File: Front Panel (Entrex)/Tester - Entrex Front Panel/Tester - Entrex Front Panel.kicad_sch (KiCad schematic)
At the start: 14 parts, among them J1 Conn_02x26_Top_Bottom, J1 Logic 8 CH, J11 Logic 8 CH, J12 Logic 8 CH, J2 Conn_01x04, J3 Conn_01x08, J4 Conn_01x08, J5 Conn_01x06, J6 Conn_01x04, J7 Conn_01x02, J8 Conn_01x19, J9 Logic 8 CH, SW1 SW_Push

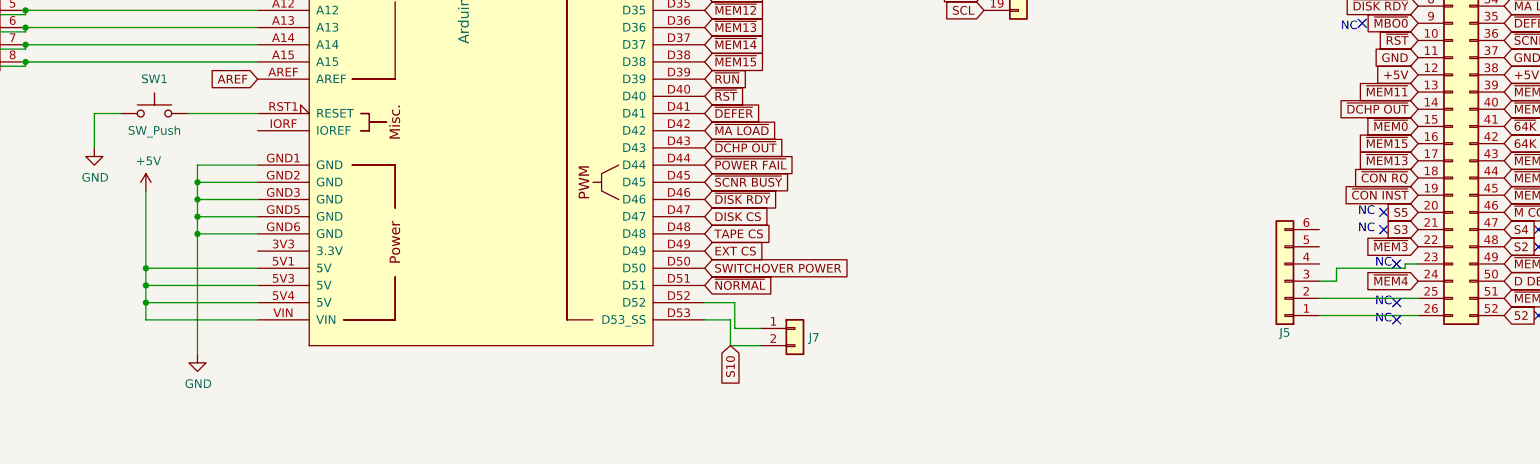
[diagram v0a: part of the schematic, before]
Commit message: build
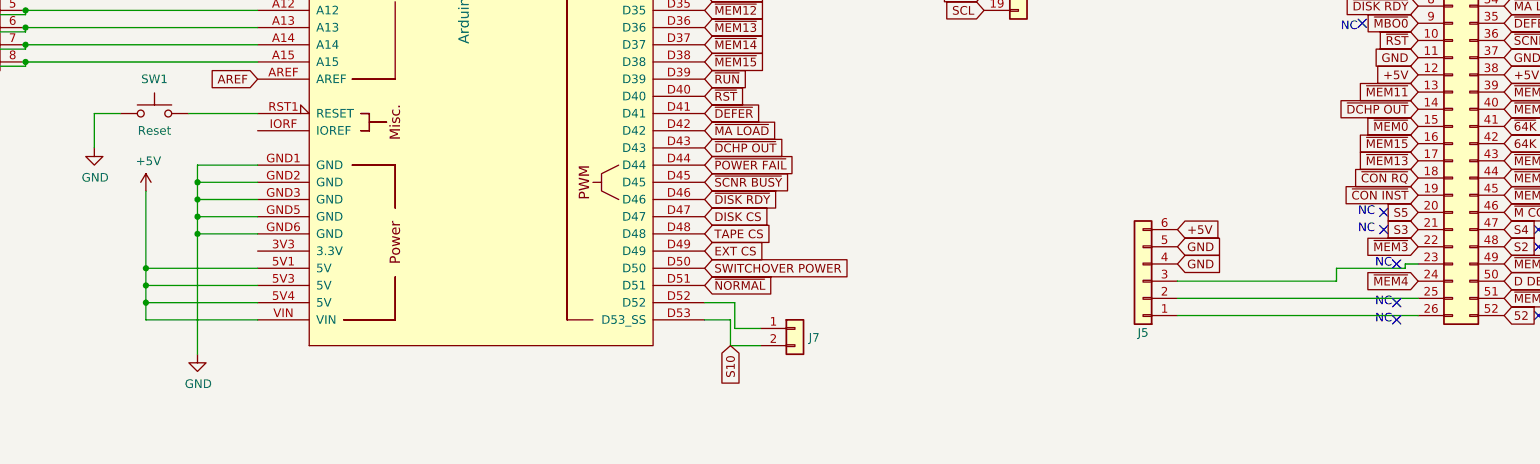
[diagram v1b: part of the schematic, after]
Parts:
- SW1: value SW_Push -> Reset
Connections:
- net +5V: now also J5.6 (Pin_6)
- net GND: now also J5.4 (Pin_4), J5.5 (Pin_5)
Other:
- moved on the sheet: J5
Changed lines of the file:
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@@
     (stroke (width 0) (type default))
   )
-  (wire (pts (xy 225.425 147.955) (xy 240.03 147.955))
+  (wire (pts (xy 204.47 147.955) (xy 240.03 147.955))
     (stroke (width 0) (type default))
   )
@@
     (stroke (width 0) (type default))
   )
-  (wire (pts (xy 227.965 145.415) (xy 225.425 145.415))
+  (wire (pts (xy 227.965 145.415) (xy 204.47 145.415))
     (stroke (width 0) (type default))
   )
@@
     (stroke (width 0) (type default))
   )
-  (wire (pts (xy 225.425 150.495) (xy 240.03 150.495))
+  (wire (pts (xy 204.47 150.495) (xy 240.03 150.495))
     (stroke (width 0) (type default))
   )
@@
     )
   )
+  (global_label "+5V" (shape input) (at 204.47 137.795 0) (fields_autoplaced)
+    (effects (font (size 1.27 1.27)) (justify left))
+    (property "Intersheetrefs" "${INTERSHEET_REFS}" (at 211.2463 137.795 0)
+      (effects (font (size 1.27 1.27)) (justify left) hide)
+    )
+  )
   (global_label "~{SCNR BUSY}" (shape input) (at 252.73 109.855 0) (fields_autoplaced)
     (effects (font (size 1.27 1.27)) (justify left))
@@
     (property "Intersheetrefs" "${INTERSHEET_REFS}" (at 165.8229 217.805 0)
       (effects (font (size 1.27 1.27)) (justify right) hide)
+    )
+  )
+  (global_label "GND" (shape input) (at 204.47 140.335 0) (fields_autoplaced)
+    (effects (font (size 1.27 1.27)) (justify left))
+    (property "Intersheetrefs" "${INTERSHEET_REFS}" (at 211.2463 140.335 0)
+      (effects (font (size 1.27 1.27)) (justify left) hide)
     )
   )
@@
     (property "Intersheetrefs" "${INTERSHEET_REFS}" (at 134.62 49.53 0)
       (effects (font (size 1.27 1.27)) hide)
+    )
+  )
+  (global_label "GND" (shape input) (at 204.47 142.875 0) (fields_autoplaced)
+    (effects (font (size 1.27 1.27)) (justify left))
+    (property "Intersheetrefs" "${INTERSHEET_REFS}" (at 211.2463 142.875 0)
+      (effects (font (size 1.27 1.27)) (justify left) hide)
     )
   )
@@
       (effects (font (size 1.27 1.27)))
     )
-    (property "Value" "SW_Push" (at 53.34 123.19 0)
+    (property "Value" "Reset" (at 53.34 123.19 0)
       (effects (font (size 1.27 1.27)))
     )
@@
     )
   )
-  (symbol (lib_id "Connector_Generic:Conn_01x06") (at 220.345 145.415 180) (unit 1)
+  (symbol (lib_id "Connector_Generic:Conn_01x06") (at 199.39 145.415 180) (unit 1)
     (in_bom yes) (on_board yes) (dnp no)
-    (property "Reference" "J5" (at 220.345 153.035 0)
+    (property "Reference" "J5" (at 199.39 153.035 0)
       (effects (font (size 1.27 1.27)))
     )
-    (property "Value" "Conn_01x06" (at 222.4278 153.6954 0)
-      (effects (font (size 1.27 1.27)) hide)
-    )
-    (property "Footprint" "port_nova:PinHeader_1x06_P2.54mm_Vertical" (at 220.345 145.415 0)
-      (effects (font (size 1.27 1.27)) hide)
-    )
-    (property "Datasheet" "~" (at 220.345 145.415 0)
-      (effects (font (size 1.27 1.27)) hide)
-    )
+    (property "Value" "Conn_01x06" (at 201.4728 153.6954 0)
+      (effects (font (size 1.27 1.27)) hide)
+    )
+    (property "Footprint" "port_nova:PinHeader_1x06_P2.54mm_Vertical" (at 199.39 145.415 0)
+      (effects (font (size 1.27 1.27)) hide)
+    )
+    (property "Datasheet" "~" (at 199.39 145.415 0)
+      (effects (font (size 1.27 1.27)) hide)
+    )
